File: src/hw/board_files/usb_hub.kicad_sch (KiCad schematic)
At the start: 5 parts, among them J1 USB_C_Receptacle_USB2.0_14P, J2 USB_A, J3 Micro_SD_Card, U3 USB2514B_Bi, U5 USB2240-AEZG-06

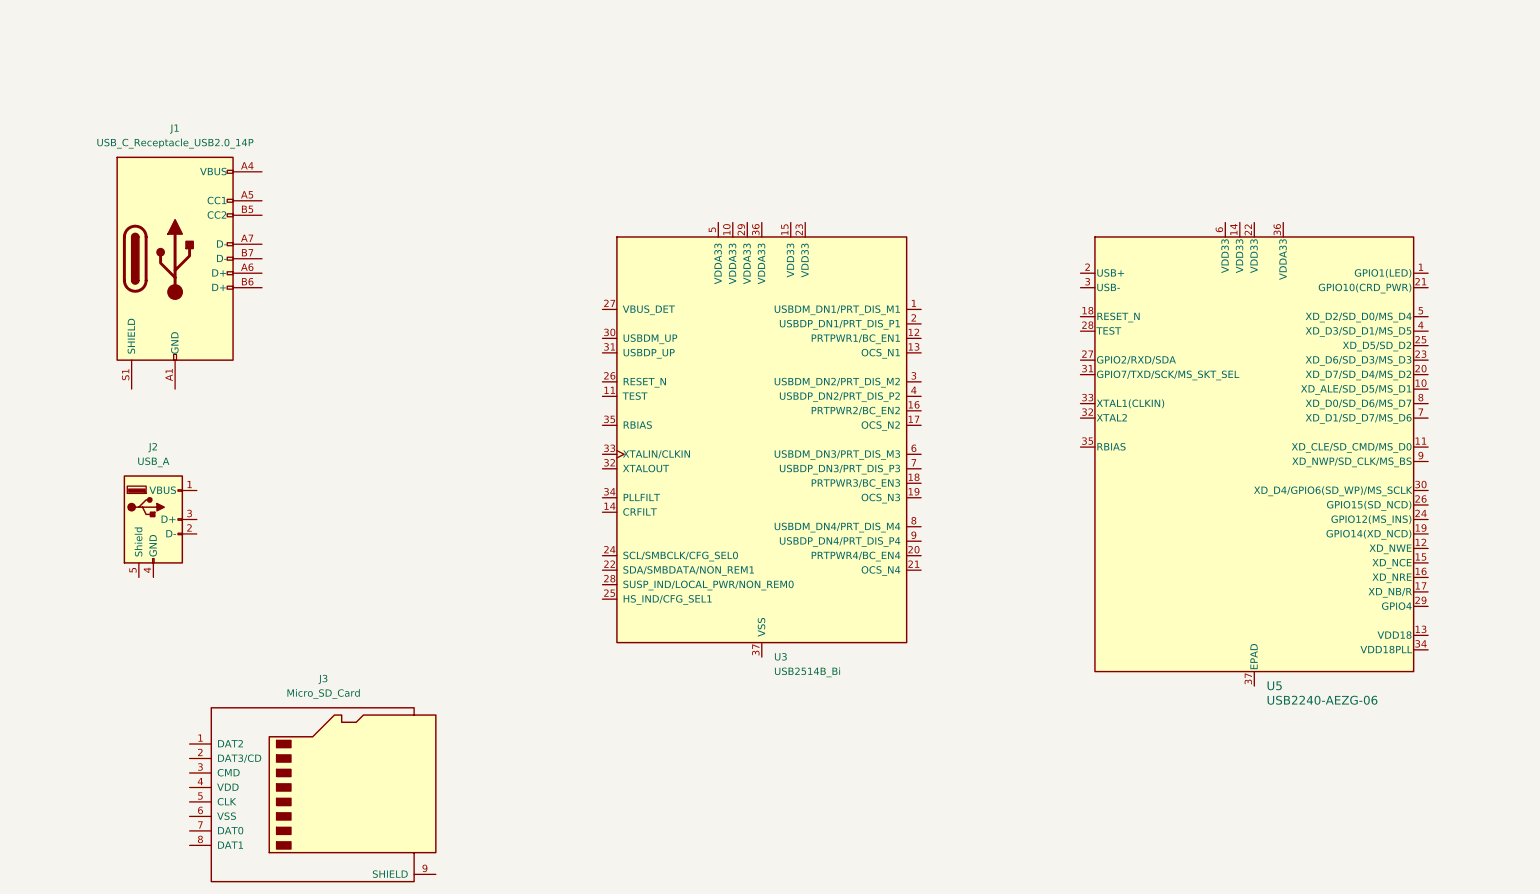
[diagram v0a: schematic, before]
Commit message: Schematic progress
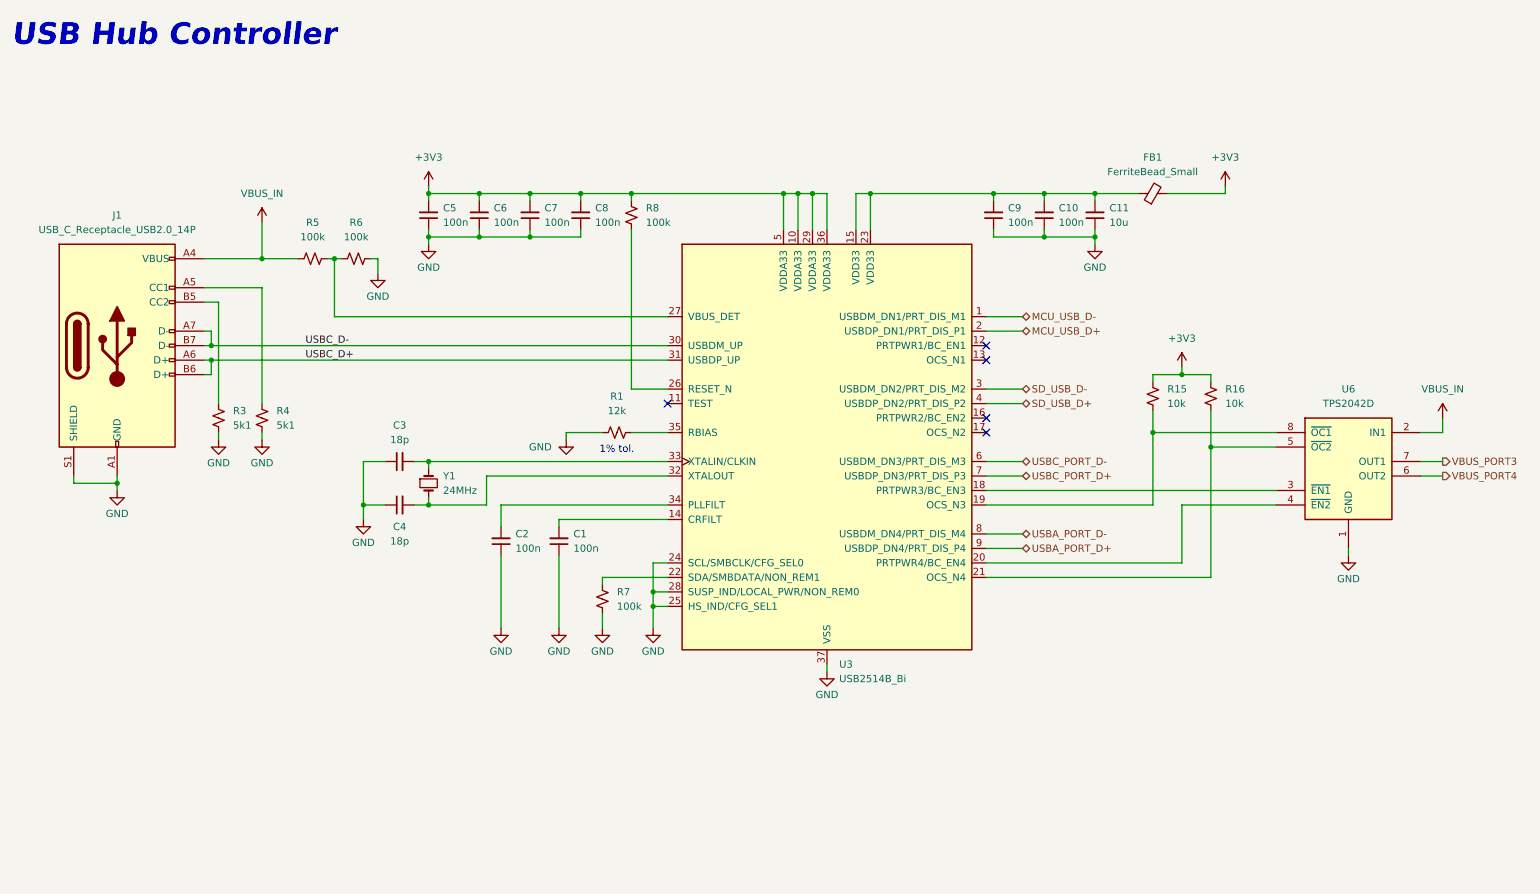
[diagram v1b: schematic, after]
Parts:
- removed J2: USB_A, symbol Connector:USB_A
- removed J3: Micro_SD_Card, symbol Connector:Micro_SD_Card
- removed U5: USB2240-AEZG-06, Package_DFN_QFN:QFN-36-1EP_6x6mm_P0.5mm_EP4.1x4.1mm_ThermalVias, symbol Project_Library:USB2240-AEZG-06
- added C1, C10, C2, C5, C6, C7, C8, C9: 100n, symbol Device:C_Small
- added C11: 10u, symbol Device:C_Small
- added C3, C4: 18p, symbol Device:C_Small
- added FB1: FerriteBead_Small, symbol Device:FerriteBead_Small
- added R1: 12k, symbol Device:R_Small_US
- added R15, R16: 10k, symbol Device:R_Small_US
- added R3, R4: 5k1, symbol Device:R_Small_US
- added R5, R6, R7, R8: 100k, symbol Device:R_Small_US
- added U6: TPS2042D, Package_SO:SOIC-8_3.9x4.9mm_P1.27mm, symbol Power_Management:TPS2042D
- added Y1: 24MHz, symbol Device:Crystal_Small
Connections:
- net MCU_USB_D-: now reaches U3.1 (USBDM_DN1/PRT_DIS_M1)
- net +3V3: now reaches U3.10 (VDDA33)
- net +3V3: now also U3.29 (VDDA33), U3.36 (VDDA33), U3.5 (VDDA33), C5.2, C6.2, C7.2, C8.2, FB1.2, R15.2, R16.2, R8.1
- net at U3.14 (CRFILT): now also C1.2
- net at U3.15 (VDD33): now also U3.23 (VDD33), C10.2, C11.2, C9.2, FB1.1
- net at U3.18 (PRTPWR3/BC_EN3): now also U6.3 (~{EN1})
- net at U3.19 (OCS_N3): now also R15.1, U6.8 (~{OC1})
- net MCU_USB_D+: now reaches U3.2 (USBDP_DN1/PRT_DIS_P1)
- net at U3.20 (PRTPWR4/BC_EN4): now also U6.4 (~{EN2})
- net at U3.21 (OCS_N4): now also R16.1, U6.5 (~{OC2})
- net at U3.22 (SDA/SMBDATA/NON_REM1): now also R7.2
- net GND: now reaches U3.24 (SCL/SMBCLK/CFG_SEL0)
- net GND: now also J1.A1 (GND), J1.A12 (GND), J1.B1 (GND), J1.B12 (GND), J1.S1 (SHIELD), U3.25 (HS_IND/CFG_SEL1), U3.28 (SUSP_IND/LOCAL_PWR/NON_REM0), U3.37 (VSS), C1.1, C10.1, C11.1, C2.1, C3.1, C4.1, C5.1, C6.1, C7.1, C8.1, C9.1, R1.1, R3.1, R4.1, R6.1, R7.1, U6.1 (GND)
- net at U3.26 (RESET_N): now also R8.2
- net at U3.27 (VBUS_DET): now also R5.1, R6.2
- net SD_USB_D-: now reaches U3.3 (USBDM_DN2/PRT_DIS_M2)
- net USBC_D-: now reaches U3.30 (USBDM_UP)
- net USBC_D-: now also J1.A7 (D-), J1.B7 (D-)
- net USBC_D+: now reaches U3.31 (USBDP_UP)
- net USBC_D+: now also J1.A6 (D+), J1.B6 (D+)
- net at U3.32 (XTALOUT): now also C4.2, Y1.2
- net at U3.33 (XTALIN/CLKIN): now also C3.2, Y1.1
- net at U3.34 (PLLFILT): now also C2.2
- net at U3.35 (RBIAS): now also R1.2
- net SD_USB_D+: now reaches U3.4 (USBDP_DN2/PRT_DIS_P2)
- net USBC_PORT_D-: now reaches U3.6 (USBDM_DN3/PRT_DIS_M3)
- net USBC_PORT_D+: now reaches U3.7 (USBDP_DN3/PRT_DIS_P3)
- net USBA_PORT_D-: now reaches U3.8 (USBDM_DN4/PRT_DIS_M4)
- net USBA_PORT_D+: now reaches U3.9 (USBDP_DN4/PRT_DIS_P4)
- net VBUS_IN: now reaches J1.A4 (VBUS), J1.A9 (VBUS), J1.B4 (VBUS), J1.B9 (VBUS)
- net VBUS_IN: now also R5.2, U6.2 (IN1)
- net at J1.A5 (CC1): now also R4.2
- net at J1.B5 (CC2): now also R3.2
- new net VBUS_PORT3: U6.7 (OUT1)
- new net VBUS_PORT4: U6.6 (OUT2)
- no-connect marks 0 -> 5
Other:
- note added: "1% tol."
- note added: "USB Hub Controller"
- moved on the sheet: J1, U3
